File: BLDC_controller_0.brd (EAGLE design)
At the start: 100 x 80 mm, 120 parts, among them IC1 78L05Z, Q10 IRF540, Q11 IRF540, Q12 IRF540, Q7 IRF540, Q8 IRF540, Q9 IRF540, T11 2N3904, T12 2N3904, T14 2N3904, T15 2N3904, T17 2N3904, T18 2N3904, T3 2N3904, T6 2N3904, T9 2N3904

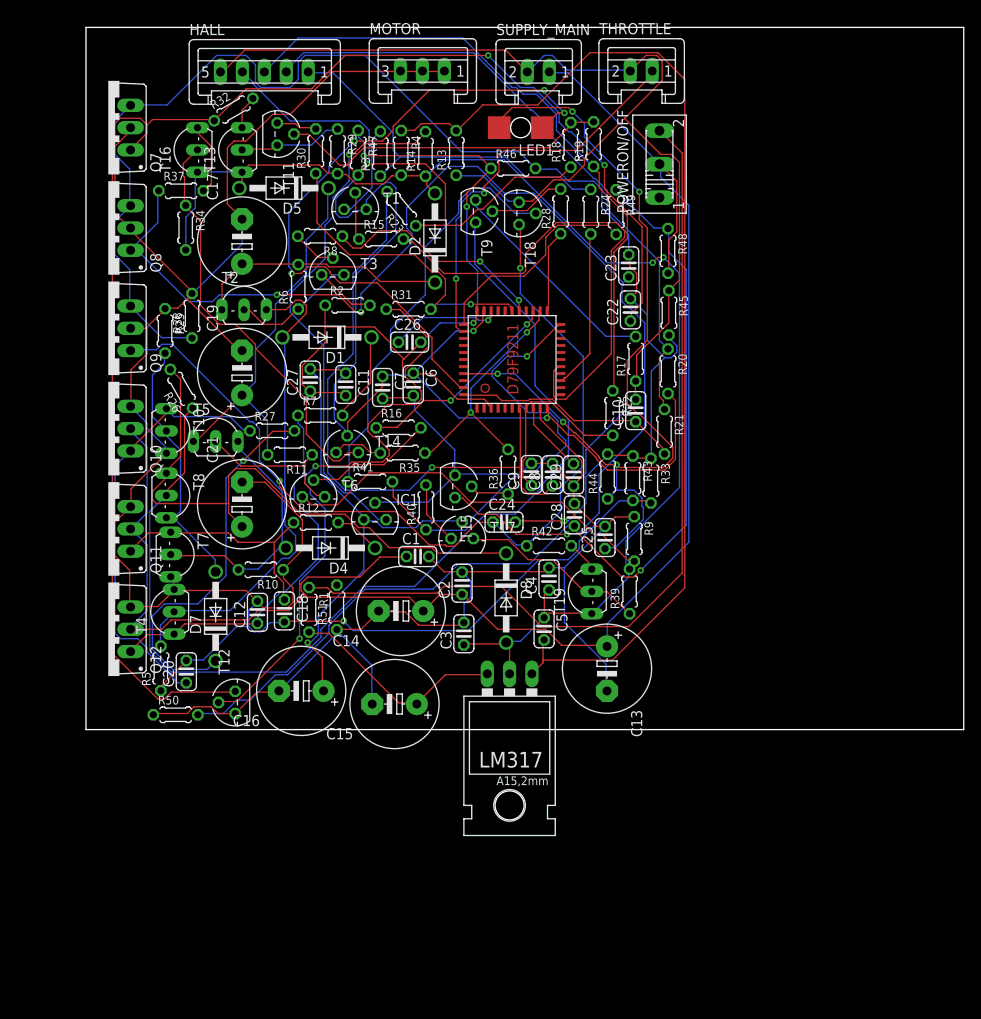
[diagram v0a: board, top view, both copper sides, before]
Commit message: Add files via upload
final bldc_motor_controller
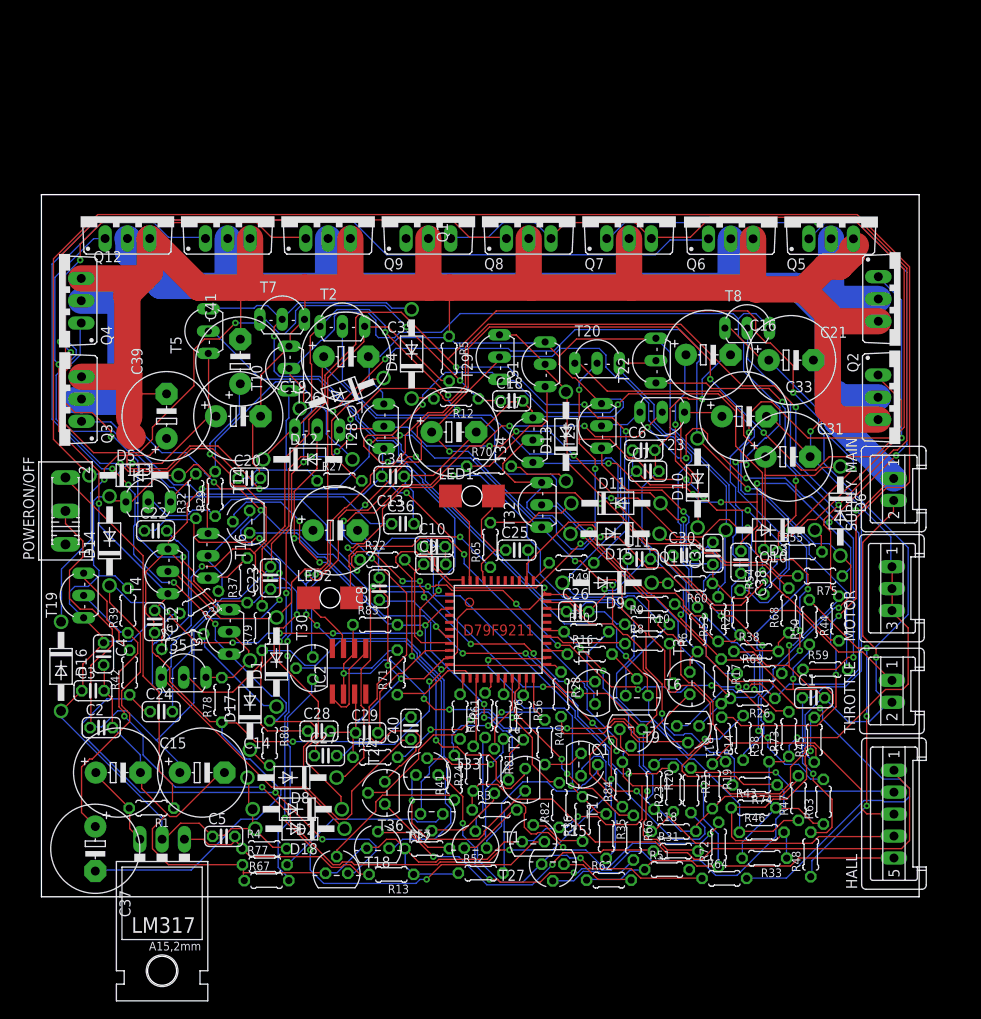
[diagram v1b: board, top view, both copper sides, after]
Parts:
- added C30, C32, C34, C36, C38, C40: 10nF, rcl:C025-024X044
- added C31, C33, C35, C37, C39, C41: 47uF, rcl:E5-10,5
- added D10, D11, D12, D13, D14, D15, D16, D17, D18, D3, D6, D9: 1N4004, diode:DO41-10
- added IC2: LM393D, linear:SO08
- added LED2: LAP4-BOTTOM, led:P47F-BOTTOM
- added Q1, Q2, Q3, Q4, Q5, Q6: IRF540, transistor-power:TO220BV
- added R52, R53, R57, R58, R62, R63, R67, R68, R72, R73, R77, R78, R82, R83: 2.2k, rcl:0204/5
- added R54, R59, R64, R69, R74, R79: 510E, rcl:0204/5
- added R55, R60, R65, R70, R75, R80: 100E, rcl:0204/5
- added R56, R61, R66, R71, R76, R81: 202k, rcl:0204/5
- added R84: 3.3k, rcl:0204/5
- added T20, T22, T23, T25, T26, T28, T29, T31, T32, T34, T35, T37: (no value), transistor-neu-to92:TO92-EBC
- added T21, T24, T27, T30, T33, T36: 2N3904, transistor:TO92
- moved HALL 110.9 mm to (97.1, 9.42), turned to 90 degrees
- moved R47 89.0 mm to (86.2, 11.2), turned to 90 degrees
- moved R13 82.5 mm to (39.9, 2.55), turned to 180 degrees
- moved R4 80.8 mm to (25.4, 5.50), turned to 0 degrees
- moved R46 80.8 mm to (82.1, 7.35)
- moved MOTOR 79.6 mm to (96.9, 35.1), turned to 90 degrees
- moved R18 79.1 mm to (72.0, 7.45), turned to 0 degrees
- moved POWERON/OFF 78.4 mm to (2.74, 44.0)
- moved T18 78.0 mm to (33.6, 2.68), turned to 0 degrees
- moved THROTTLE 76.2 mm to (96.9, 23.4), turned to 90 degrees
- moved R3 75.9 mm to (51.6, 9.90), turned to 0 degrees
- moved R14 75.7 mm to (80.0, 18.1)
- moved R38 74.8 mm to (81.4, 27.9), turned to 0 degrees
- moved R19 74.4 mm to (76.5, 12.6), turned to 270 degrees
- moved T1 74.0 mm to (49.5, 5.56)
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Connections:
- new net N$101: R72.2, T33.3
- new net N$102: R74.1, T32.B, T33.1
- new net N$103: R76.2, T33.2
- new net N$104: D15.A, R73.2, T32.C, T34.B
- new net N$105: D15.C, R75.2
- new net N$106: C38.1, Q5.G, R75.1, T34.E
- new net N$107: C39.+, D16.C, R74.2, T32.E
- new net N$109: R77.2, T36.3
- new net N$110: R79.1, T35.B, T36.1
- new net N$111: R81.2, T36.2
- new net N$112: D17.A, R78.2, T35.C, T37.B
- new net N$113: D17.C, R80.2
- new net N$114: C40.1, Q6.G, R80.1, T37.E
- new net N$115: C41.+, D18.C, R79.2, T35.E
- new net N$117: R61.1, U$1.B0
- new net N$118: R71.1, U$1.B1
- new net N$119: R81.1, U$1.B7
- new net N$120: R76.1, U$1.B6
- new net N$121: R66.1, U$1.B8
- new net N$122: R56.1, U$1.B9
- new net N$123: IC2.1, IC2.5
- new net N$124: IC2.2, IC2.6, R82.2, R83.1
- new net N$125: LED2.C, R84.1
- new net N$126: IC2.7, LED2.A
- new net N$19: R57.2, T24.3
- new net N$69: R52.2, T21.3
- new net N$70: R54.1, T20.B, T21.1
- new net N$71: R56.2, T21.2
- new net N$72: D3.A, R53.2, T20.C, T22.B
- new net N$73: D3.C, R55.2
- new net N$74: C30.1, Q1.G, R55.1, T22.E
- new net N$75: C31.+, D6.C, R54.2, T20.E
- new net N$78: R59.1, T23.B, T24.1
- new net N$79: R61.2, T24.2
- new net N$80: D9.A, R58.2, T23.C, T25.B
- new net N$81: D9.C, R60.2
- new net N$82: C32.1, Q2.G, R60.1, T25.E
- new net N$83: C33.+, D10.C, R59.2, T23.E
- new net N$85: R62.2, T27.3
- new net N$86: R64.1, T26.B, T27.1
- new net N$87: R66.2, T27.2
- new net N$88: D11.A, R63.2, T26.C, T28.B
- new net N$89: D11.C, R65.2
- new net N$90: C34.1, Q3.G, R65.1, T28.E
- new net N$91: C35.+, D12.C, R64.2, T26.E
- new net N$93: R67.2, T30.3
- new net N$94: R69.1, T29.B, T30.1
- new net N$95: R71.2, T30.2
- new net N$96: D13.A, R68.2, T29.C, T31.B
- new net N$97: D13.C, R70.2
- new net N$98: C36.1, Q4.G, R70.1, T31.E
- new net N$99: C37.+, D14.C, R69.2, T29.E
- new net V+: IC2.8
- new net V-: IC2.4
- net +15V: now also D10.A, D12.A, D14.A, D16.A, D18.A, D6.A
- net +5V: now also R83.2
- net 0V: now also IC2.3, R52.1, R57.1, R62.1, R67.1, R72.1, R77.1, R82.1, R84.2
- net MOTOR_U: now also C30.2, C31.-, C32.2, C33.-, C34.2, C35.-, C36.2, C37.-, C38.2, C39.-, C40.2, C41.-, Q1.S, Q2.S, Q3.S, Q4.S, Q5.S, Q6.S, R53.1, R58.1, R63.1, R68.1, R73.1, R78.1, T22.C, T25.C, T28.C, T31.C, T34.C, T37.C
- net VPP: now also Q1.D, Q2.D, Q3.D, Q4.D, Q5.D, Q6.D
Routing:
- net MOTOR_U: track 238.5 -> 581.6 mm, vias 1 -> 4
- net N$99: track 0.00 -> 188.4 mm, vias 0 -> 12
- net N$35: track 43.4 -> 223.2 mm, vias 0 -> 3
- net N$114: track 0.00 -> 177.6 mm, vias 0 -> 4
- net VPP: track 191.5 -> 335.4 mm, vias 0 -> 6
- net N$59: track 161.8 -> 303.8 mm, vias 1 -> 8
- net N$78: track 0.00 -> 139.2 mm, vias 0 -> 8
- net N$91: track 0.00 -> 131.1 mm, vias 0 -> 2
- net N$107: track 0.00 -> 130.2 mm, vias 0 -> 6
- net N$30: track 112.7 -> 237.0 mm, vias 1 -> 9
- net N$70: track 0.00 -> 121.3 mm, vias 0 -> 8
- net N$102: track 0.00 -> 113.4 mm, vias 0 -> 4
- net N$94: track 0.00 -> 109.7 mm, vias 0 -> 1
- net +15V: track 144.0 -> 246.8 mm, vias 2 -> 4
- net N$106: track 0.00 -> 100.1 mm, vias 0 -> 6
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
